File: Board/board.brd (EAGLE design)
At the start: 78.7 x 73.7 mm, 23 parts, among them IC1 L293D, U1 ARDUINOR3-BPLACE

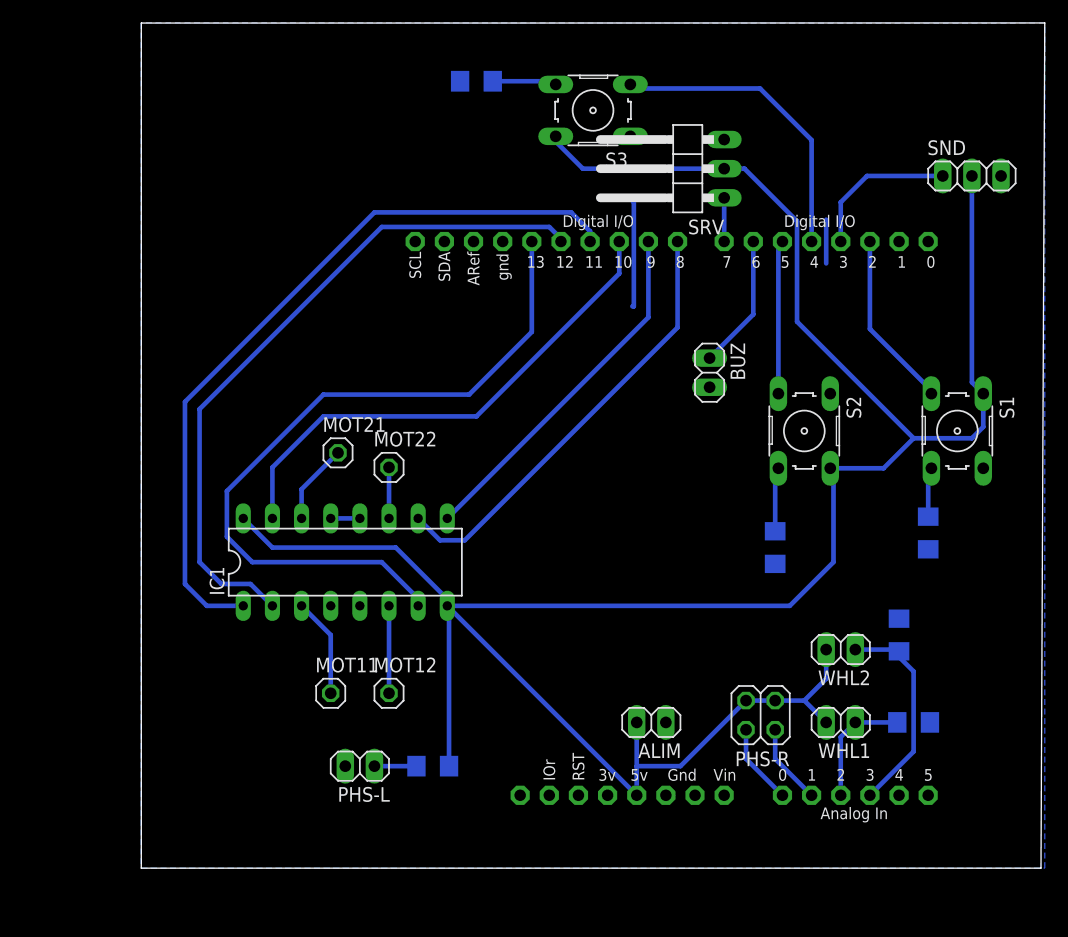
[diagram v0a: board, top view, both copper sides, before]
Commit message: Board preparation
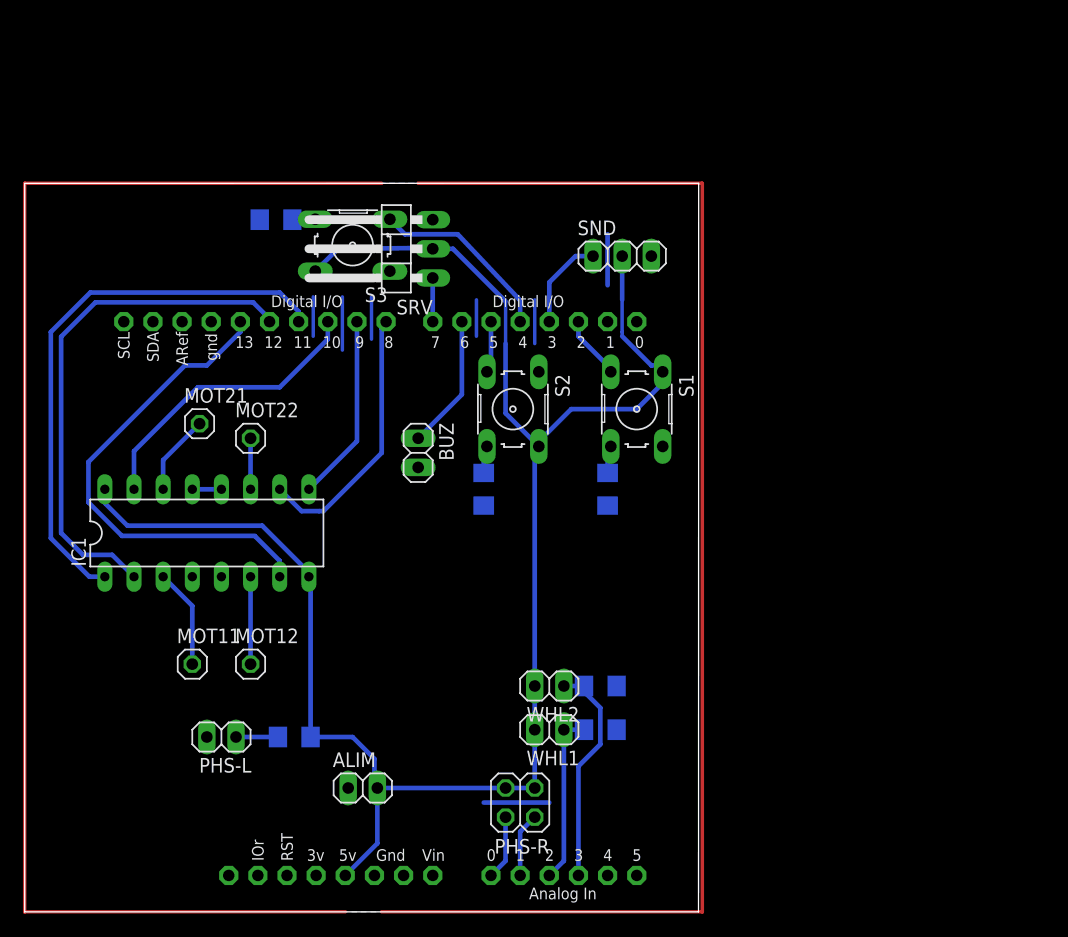
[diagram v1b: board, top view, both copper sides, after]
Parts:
- moved SND 31.3 mm to (52.1, 57.1)
- moved R1 28.2 mm to (50.8, 36.8)
- moved S1 28.0 mm to (53.3, 43.8)
- moved R4 27.3 mm to (50.2, 15.9)
- moved R5 26.4 mm to (50.2, 19.7), turned to 180 degrees
- moved BUZ 26.3 mm to (34.3, 40.0)
- moved SRV 26.3 mm to (31.8, 57.8)
- moved U1 26.3 mm to (-10.2, 0.64)
- moved R2 25.9 mm to (40.0, 36.8)
- moved ALIM 25.8 mm to (29.5, 10.8), turned to 0 degrees
- moved WHL2 25.6 mm to (45.7, 19.7)
- moved S2 25.5 mm to (42.5, 43.8)
- moved WHL1 25.4 mm to (45.7, 15.9)
- moved S3 24.0 mm to (28.6, 58.1)
- moved PHS-R 22.3 mm to (43.2, 9.53)
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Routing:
- net N$5: track 0.00 -> 122.6 mm
- net N$6: track 0.00 -> 116.2 mm
- net +5V: track 217.8 -> 156.5 mm
- net PIN13: track 63.7 -> 42.5 mm
- net N$7: track 44.5 -> 25.8 mm
- net N$10: track 65.5 -> 48.7 mm
- net GND: track 16.4 -> 32.1 mm
- net N$9: track 38.6 -> 23.4 mm
- net N$8: track 31.4 -> 16.3 mm
- net PIN12: track 60.0 -> 45.3 mm
- net PIN4: track 26.7 -> 16.2 mm
- net PIN2: track 15.5 -> 5.54 mm
- net PIN5: track 13.4 -> 4.52 mm
- net N$22: track 13.3 -> 8.18 mm
- net N$11: track 10.5 -> 15.0 mm
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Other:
- board size 78.7 x 73.7 mm -> 58.7 x 63.5 mm
